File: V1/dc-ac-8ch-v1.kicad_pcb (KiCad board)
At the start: 2 copper layers, 98 x 67.8 mm, 100 parts, among them J1 DB142V-5.08-8P, J2 DB142V-5.08-2P, J4 DB142V-5.08-2P, U1 MOC3063S, U2 MOC3063S, U3 MOC3063S, U4 MOC3063S, U5 MOC3063S, U6 MOC3063S, U7 MOC3063S, U8 MOC3063S

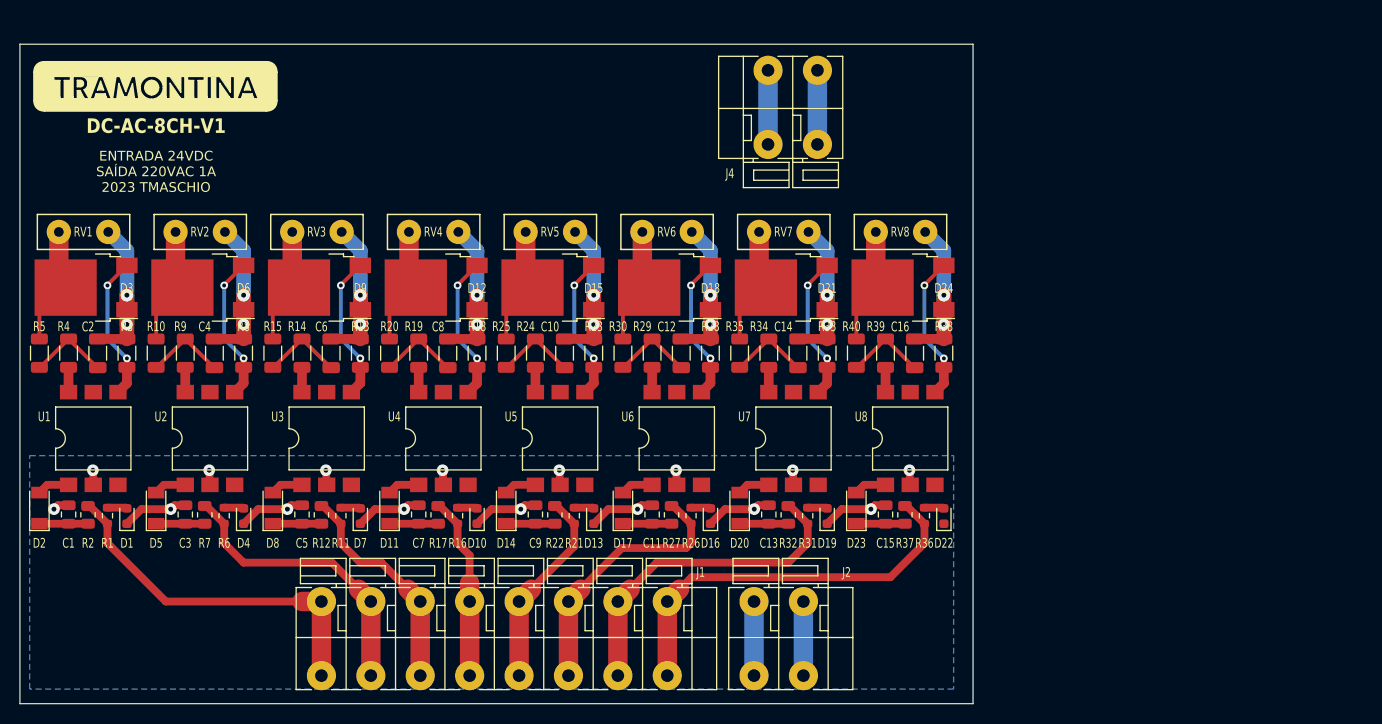
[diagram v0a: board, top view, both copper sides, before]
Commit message: Development
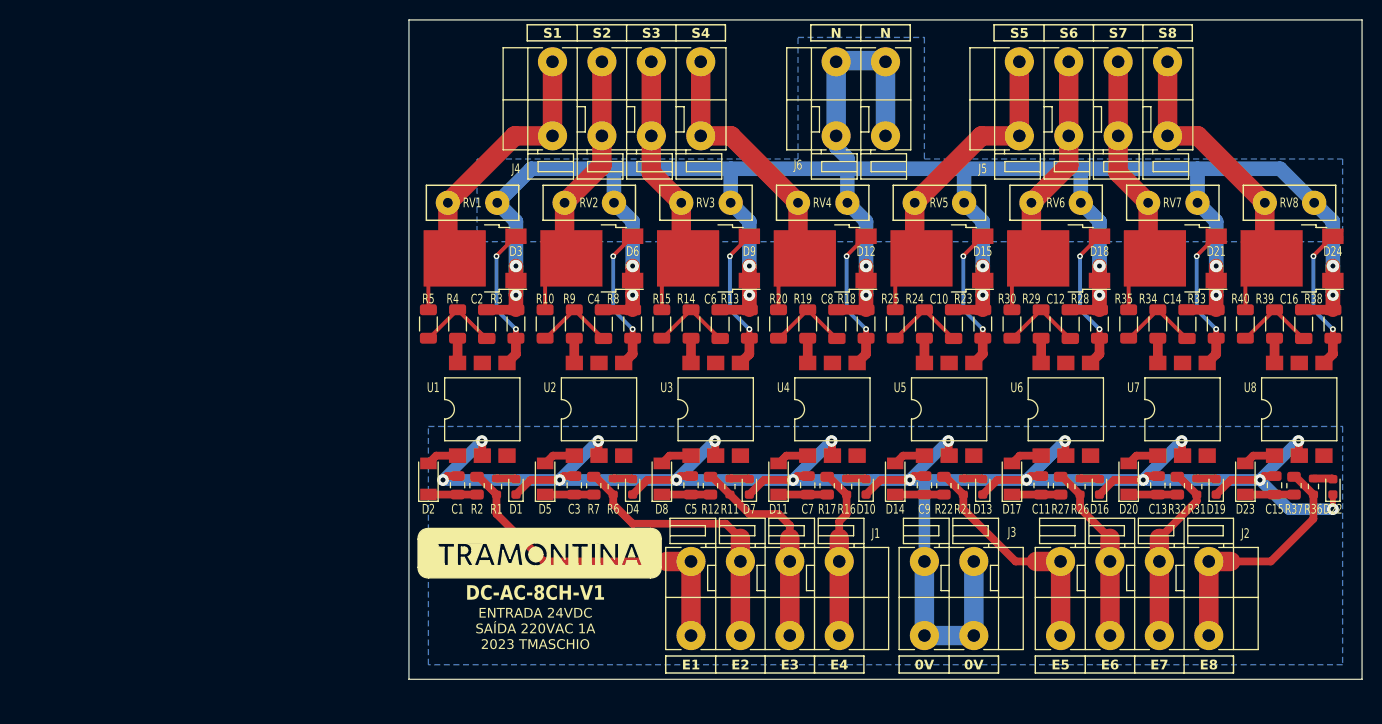
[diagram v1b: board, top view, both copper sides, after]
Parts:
- removed the REF** at (74.0, 69.0)
- added J2: DB142V-5.08-4P, Tales:TerminalBlock_Dibo_DB142V-5.08-4P_1x04_P5.08mm_Vertical_copy, F.Cu at (167.0, 125.5)
- added J4: DB142V-5.08-4P, Tales:TerminalBlock_Dibo_DB142V-5.08-4P_1x04_P5.08mm_Vertical_copy, F.Cu at (130.0, 66.5)
- added J5: DB142V-5.08-4P, Tales:TerminalBlock_Dibo_DB142V-5.08-4P_1x04_P5.08mm_Vertical_copy, F.Cu at (178.0, 66.5)
- added REF**: Logo_Tramontina_25mm_Silk, Tales:Logo_Tramontina_25mm_Silk, F.Cu at (113.5, 117.0)
- J1: value DB142V-5.08-8P -> DB142V-5.08-4P; footprint Tales:TerminalBlock_Dibo_DB142V-5.08-8P_1x08_P5.08mm_Vertical -> Tales:TerminalBlock_Dibo_DB142V-5.08-4P_1x04_P5.08mm_Vertical_copy
- moved D12 40.1 mm to (142.8, 86.7)
- moved D15 40.1 mm to (154.8, 86.7)
- moved D18 40.1 mm to (166.8, 86.7)
- moved D9 40.1 mm to (130.8, 86.7)
- moved C1 40.1 mm to (105.0, 110.0)
- moved C10 40.1 mm to (156.0, 93.5)
- moved C11 40.1 mm to (165.0, 110.0)
- moved C12 40.1 mm to (168.0, 93.5)
- moved C13 40.1 mm to (177.0, 110.0)
- moved C14 40.1 mm to (180.0, 93.5)
- moved C15 40.1 mm to (189.0, 110.0)
- moved C16 40.1 mm to (192.0, 93.5)
- moved C2 40.1 mm to (108.0, 93.5)
- moved C3 40.1 mm to (117.0, 110.0)
- moved C4 40.1 mm to (120.0, 93.5)
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- renumbered J2 to J3, J4 to J6
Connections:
- R21 pad 1: Net-(J1-Pin_5) -> Net-(J2-Pin_1)
- R22 pad 2: Net-(J1-Pin_5) -> Net-(J2-Pin_1)
- R26 pad 1: Net-(J1-Pin_6) -> Net-(J2-Pin_2)
- R27 pad 2: Net-(J1-Pin_6) -> Net-(J2-Pin_2)
- R31 pad 1: Net-(J1-Pin_7) -> Net-(J2-Pin_3)
- R32 pad 2: Net-(J1-Pin_7) -> Net-(J2-Pin_3)
- R36 pad 1: Net-(J1-Pin_8) -> Net-(J2-Pin_4)
- R37 pad 2: Net-(J1-Pin_8) -> Net-(J2-Pin_4)
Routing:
- net GND: track 76.5 -> 229.4 mm, vias 16 -> 17
- net NEUTRAL: track 157.6 -> 274.9 mm
- net Net-(J1-Pin_8): track 41.3 -> 0.00 mm
- net Net-(J1-Pin_7): track 34.4 -> 0.00 mm
- net Net-(J1-Pin_6): track 27.5 -> 0.00 mm
- net Net-(J2-Pin_4): track 0.00 -> 25.5 mm
- net Net-(J2-Pin_1): track 0.00 -> 24.1 mm
- net Net-(D3-A2): track 12.4 -> 33.6 mm
- net Net-(D15-A2): track 12.4 -> 33.6 mm
- net Net-(J1-Pin_5): track 20.7 -> 0.00 mm
- net Net-(D24-A2): track 12.4 -> 32.9 mm
- net Net-(D12-A2): track 12.4 -> 32.9 mm
- net Net-(J2-Pin_3): track 0.00 -> 18.8 mm
- net Net-(J2-Pin_2): track 0.00 -> 18.5 mm
- net Net-(D6-A2): track 12.4 -> 28.5 mm
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- added copper zone on B.Cu, net NEUTRAL
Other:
- board text added: "0V"
- board text added: "E1"
- board text added: "E2"
- board text added: "E3"
- board text added: "E4"
- board text added: "E5"
- board text added: "E6"
- board text added: "E7"
- board text added: "E8"
- board text added: "N"
- board text added: "S1"
- board text added: "S2"
- board text added: "S3"
- board text added: "S4"
- board text added: "S5"
- board text added: "S6"
- board text added: "S7"
- board text added: "S8"
- board text added: "SUPORTES PCI METALTEX SP7 1x pé macho 9 mm 1x pé fêmea 9 mm 2x espaçadores 30 mm 1x espaçador 20 mm Comprimento total 98 mm Largura da placa 67,8 mm"
- board text removed: "SUPORTES PCI METALTEX SP7 1x pé macho 9 mm 1x pé fêmea 9 mm 2x espaçadores 45 mm Comprimento total 108 mm Largura da placa 67,8 mm"
